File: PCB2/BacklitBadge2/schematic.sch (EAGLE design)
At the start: 35 parts

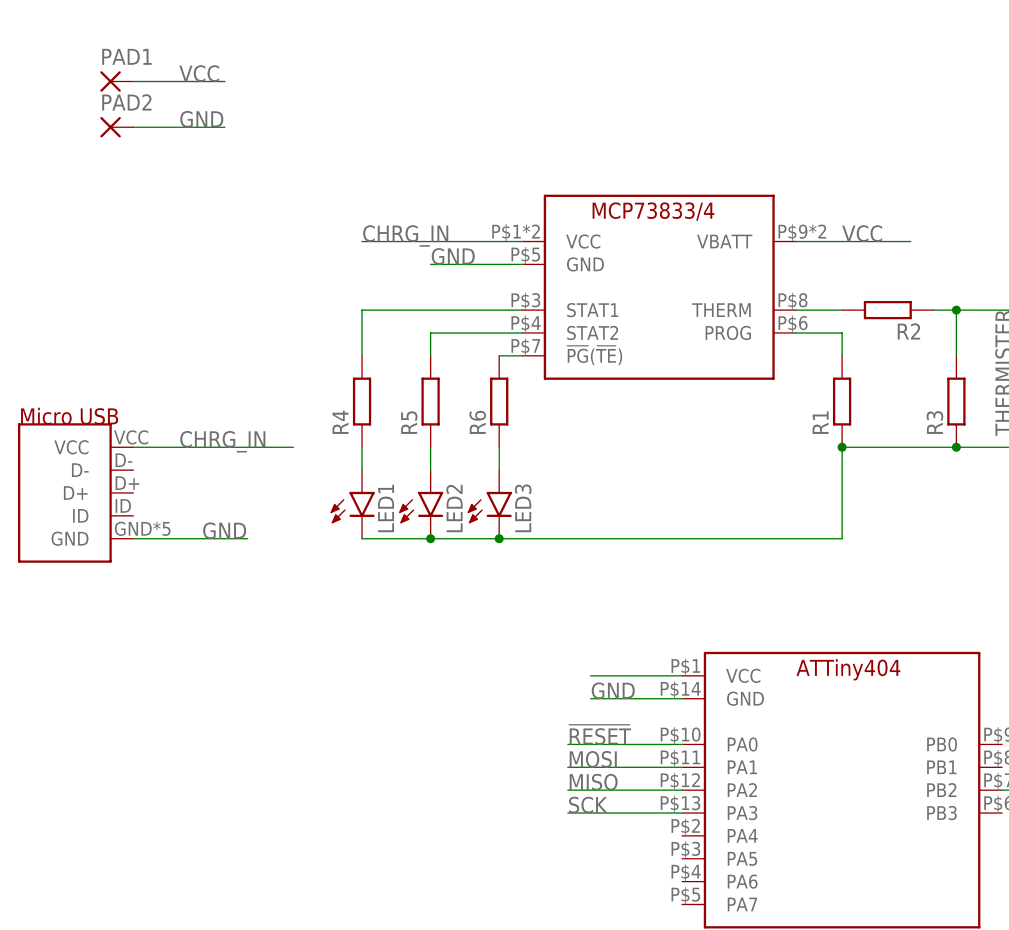
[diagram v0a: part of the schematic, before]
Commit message: Updates to the schematic
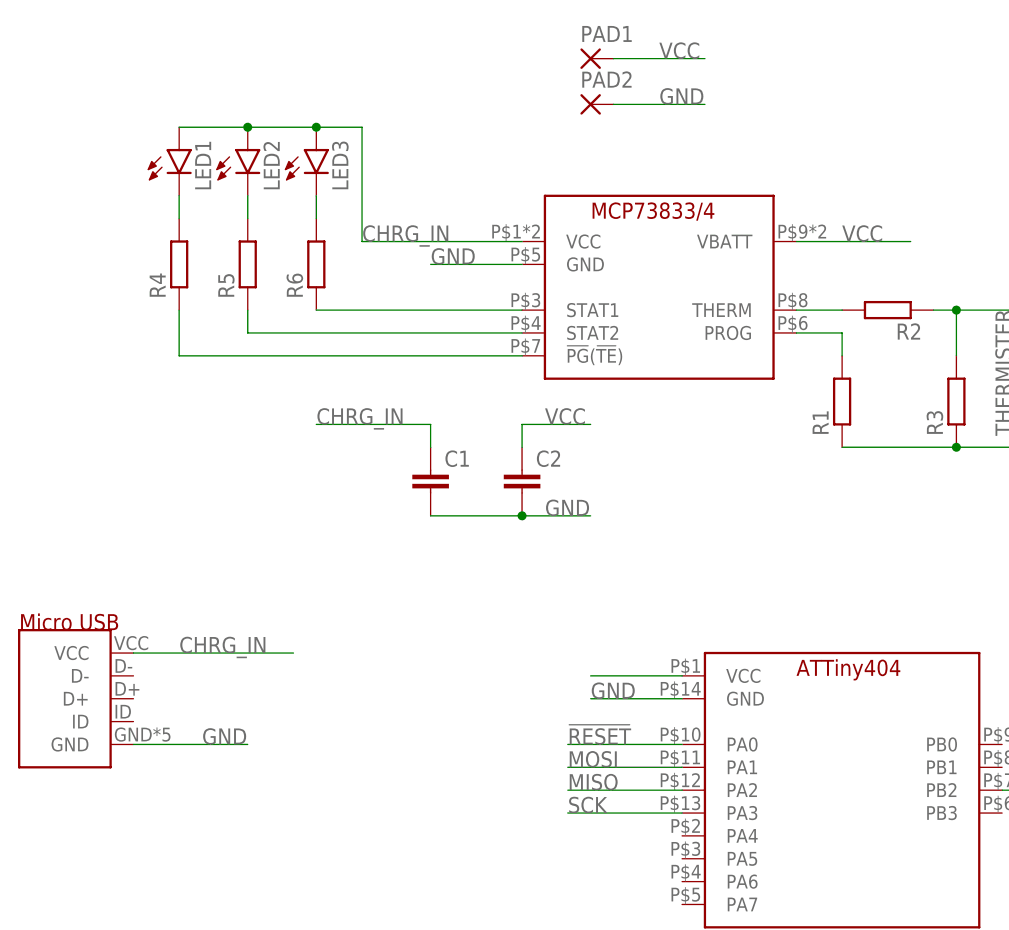
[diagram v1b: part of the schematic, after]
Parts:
- added C1, C2: (no value), eagle-ltspice:CC1206
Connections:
- removed net N$30: R5.2, U$2.STAT2
- new net N$9: LED3.C, R6.2
- net CHRG_IN: now also C1.1, LED1.A, LED2.A, LED3.A
- net GND: now also C1.2, C2.2; no longer LED1.C, LED2.C, LED3.C
- net N$14: now also R5.1, U$2.STAT2; no longer LED1.A, R4.1
- net N$28: now also R4.1; no longer R6.2
- net N$6: now also LED1.C, R4.2; no longer LED3.A, R6.1
- net N$7: now also LED2.C, R5.2; no longer LED2.A, R5.1
- net N$8: now also R6.1; no longer R4.2
- net VCC: now also C2.1
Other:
- moved on the sheet: LED1, LED2, LED3, PAD1, PAD2, R4, R5, R6
